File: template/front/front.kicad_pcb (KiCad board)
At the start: 2 copper layers, 30.5 x 99.1 mm, 3 parts, among them J1 PinHeader_02x04_P2.54_THT_ang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

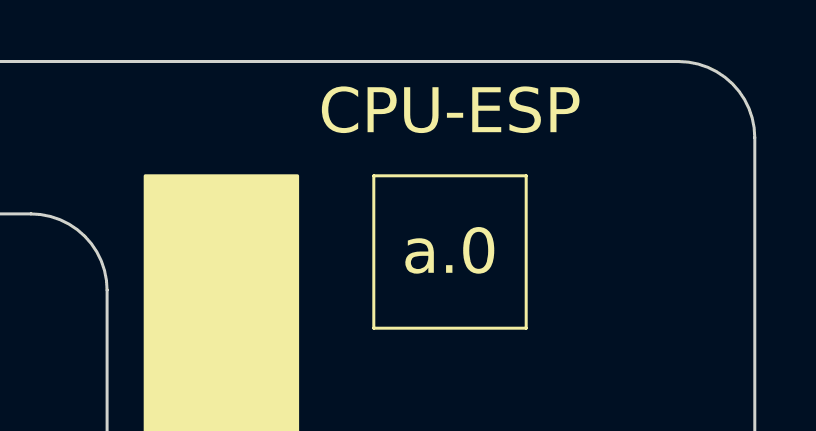
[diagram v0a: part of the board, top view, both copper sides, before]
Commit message: PM-PS
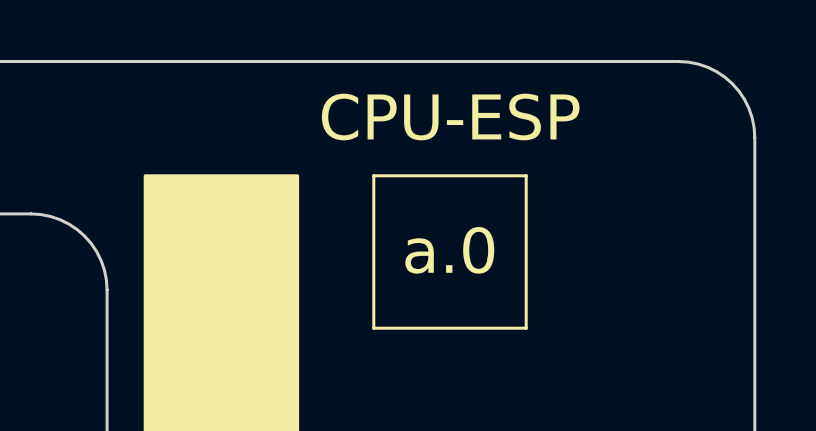
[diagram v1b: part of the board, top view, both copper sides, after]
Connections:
- net +5V renamed +3.3V
- J1 pad 3: unconnected-(J1-Pin_3-Pad3) -> /MOSI
- J1 pad 4: unconnected-(J1-Pin_4-Pad4) -> /SCK
- J1 pad 5: unconnected-(J1-Pin_5-Pad5) -> /MISO
- J1 pad 6: unconnected-(J1-Pin_6-Pad6) -> /CS
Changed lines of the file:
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@@
 	(net 0 "")
 	(net 1 "GND")
-	(net 2 "unconnected-(J1-Pin_6-Pad6)")
-	(net 3 "+5V")
-	(net 4 "unconnected-(J1-Pin_4-Pad4)")
-	(net 5 "unconnected-(J1-Pin_5-Pad5)")
-	(net 6 "unconnected-(J1-Pin_3-Pad3)")
+	(net 2 "+3.3V")
+	(net 3 "/CS")
+	(net 4 "/MISO")
+	(net 5 "/SCK")
+	(net 6 "/MOSI")
 	(footprint "Symbol:OSHW-Symbol_6.7x6mm_SilkScreen"
 		(layer "B.Cu")
@@
 			(layers "*.Cu" "*.Mask")
 			(remove_unused_layers no)
-			(net 3 "+5V")
+			(net 2 "+3.3V")
 			(pinfunction "Pin_1")
 			(pintype "passive")
@@
 			(layers "*.Cu" "*.Mask")
 			(remove_unused_layers no)
-			(net 3 "+5V")
+			(net 2 "+3.3V")
 			(pinfunction "Pin_2")
 			(pintype "passive")
@@
 			(layers "*.Cu" "*.Mask")
 			(remove_unused_layers no)
-			(net 6 "unconnected-(J1-Pin_3-Pad3)")
+			(net 6 "/MOSI")
 			(pinfunction "Pin_3")
-			(pintype "passive+no_connect")
+			(pintype "passive")
 		)
 		(pad "4" thru_hole oval
@@
 			(layers "*.Cu" "*.Mask")
 			(remove_unused_layers no)
-			(net 4 "unconnected-(J1-Pin_4-Pad4)")
+			(net 5 "/SCK")
 			(pinfunction "Pin_4")
-			(pintype "passive+no_connect")
+			(pintype "passive")
 		)
 		(pad "5" thru_hole oval
@@
 			(layers "*.Cu" "*.Mask")
 			(remove_unused_layers no)
-			(net 5 "unconnected-(J1-Pin_5-Pad5)")
+			(net 4 "/MISO")
 			(pinfunction "Pin_5")
-			(pintype "passive+no_connect")
+			(pintype "passive")
 		)
 		(pad "6" thru_hole oval
@@
 			(layers "*.Cu" "*.Mask")
 			(remove_unused_layers no)
-			(net 2 "unconnected-(J1-Pin_6-Pad6)")
+			(net 3 "/CS")
 			(pinfunction "Pin_6")
-			(pintype "passive+no_connect")
+			(pintype "passive")
 		)
 		(pad "7" thru_hole oval
@@
 	)
 	(gr_line
+		(start 70.485 49.53)
+		(end 70.485 44.45)
+		(stroke
+			(width 0.1)
+			(type default)
+		)
+		(layer "Cmts.User")
+	)
+	(gr_line
 		(start 88.9 100.33)
 		(end 52.07 100.33)
@@
 	)
 	(gr_text "CPU-ESP"
-		(at 71.12 53.34 0)
+		(at 71.12 52.705 0)
 		(layer "F.SilkS")
 		(effects
@@
 				(thickness 0.2)
 			)
-			(justify bottom)
-		)
-	)
+		)
+	)
